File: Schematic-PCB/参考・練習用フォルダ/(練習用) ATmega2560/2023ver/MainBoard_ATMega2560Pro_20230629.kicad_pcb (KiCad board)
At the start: 2 copper layers, 70 x 103 mm, 43 parts, among them J1 Conn_01x10_Pin, J2 Conn_01x08_Male, J3 Conn_01x04_Female, J4 Conn_01x08_Male, J5 Conn_01x02_Male, J6 Conn_01x20_Male, J7 Conn_01x26_Male, J8 Conn_01x03_Pin, SW1 SW_DPST_x2, SW2 SW_DPST_x2, SW3 SW_DPST_x2, SW4 SW_DPDT_x2, U1 ATMEGA2560_pro

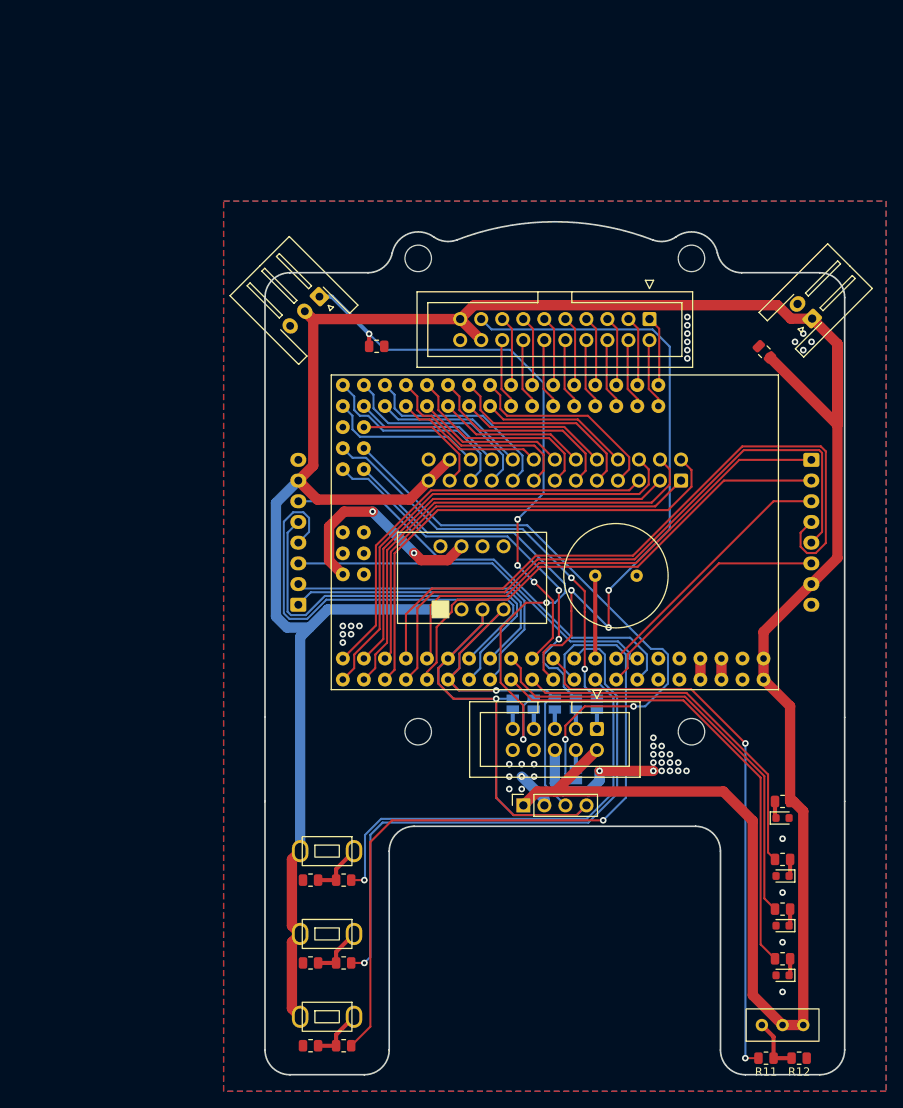
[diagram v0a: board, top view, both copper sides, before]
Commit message: update: いろいろなKiCadファイルを開いた
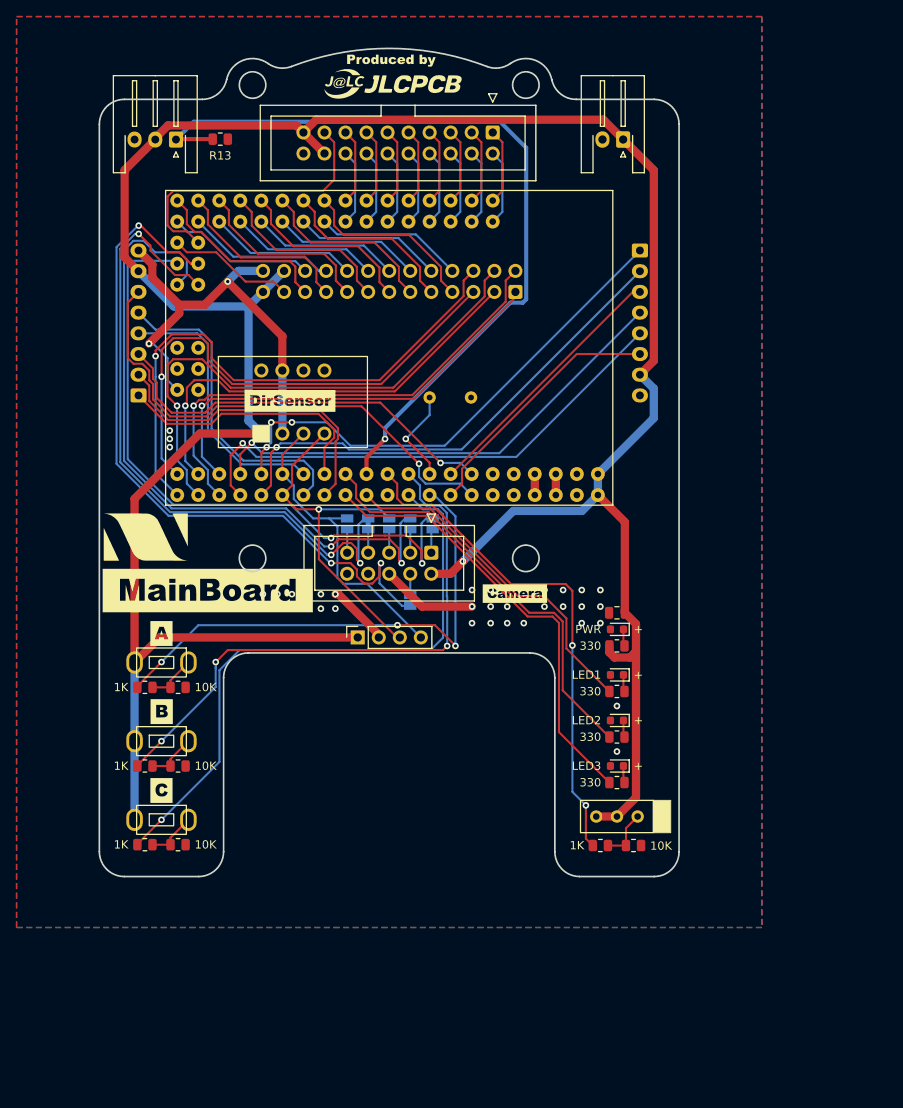
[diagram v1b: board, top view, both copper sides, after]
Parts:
- removed D1, D2, D3, D4: LED, LED_SMD:LED_0603_1608Metric
- removed REF** (x4): MountingHole_3.2mm_M3, MountingHole:MountingHole_3.2mm_M3
- added LED1: LED, LED_SMD:LED_0603_1608Metric, F.Cu at (112.5, 119.5)
- added LED2: LED, LED_SMD:LED_0603_1608Metric, F.Cu at (112.5, 125.0)
- added LED3: LED, LED_SMD:LED_0603_1608Metric, F.Cu at (112.5, 130.5)
- added PWR: LED, LED_SMD:LED_0603_1608Metric, F.Cu at (112.5, 114.0)
- BZ1: moved to B.Cu
- JP3: value Jumper_2_Open -> Jumper_2_Bridged; footprint Jumper:SolderJumper-2_P1.3mm_Open_Pad1.0x1.5mm -> Jumper:SolderJumper-2_P1.3mm_Bridged_Pad1.0x1.5mm
- moved C1 36.2 mm to (112.5, 112.0), turned to 180 degrees
- moved R9 34.1 mm to (55.5, 140.0), turned to 180 degrees
- moved R7 33.8 mm to (55.5, 130.5), turned to 180 degrees
- moved R5 33.4 mm to (55.5, 121.0), turned to 180 degrees
- moved J4 32.7 mm to (115.3, 68.2)
- moved R11 32.5 mm to (110.5, 140.1)
- moved R12 32.5 mm to (114.5, 140.1)
- moved SW4 32.2 mm to (112.5, 136.6), turned to 0 degrees
- moved J2 31.8 mm to (54.7, 85.8)
- moved J5 31.4 mm to (113.2, 54.9), turned to 180 degrees
- moved R13 31.3 mm to (64.6, 54.8)
- moved SW3 31.1 mm to (57.5, 137.0)
- moved SW2 30.7 mm to (57.5, 127.5)
- moved J7 30.3 mm to (100.2, 73.3)
- moved SW1 30.3 mm to (57.5, 118.0)
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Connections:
- U1 pad D11: Sig_NeoPixel -> unconnected-(U1-PadD11)
- U1 pad D48: unconnected-(U1-PadD48) -> Sig23_BALL-Kicker
- U1 pad D49: Sig23_BALL-Kicker -> Sig_NeoPixel
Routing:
- net VIN: track 376.9 -> 325.1 mm, vias 0 -> 1
- net SDA: track 88.2 -> 37.6 mm, vias 1 -> 0
- net Sig_NeoPixel: track 80.9 -> 35.2 mm, vias 3 -> 0
- net SCK: track 48.4 -> 84.4 mm
- net MISO: track 50.0 -> 77.9 mm
- net Sig_Kicker: track 70.3 -> 97.2 mm, vias 4 -> 1
- net GND: track 48.9 -> 74.2 mm, vias 46 -> 38
- net Sig_M4-1: track 83.1 -> 58.8 mm, vias 0 -> 1
- net Sig_M2-1: track 56.3 -> 33.1 mm
- net SS: track 60.9 -> 81.0 mm, vias 2 -> 3
- net Sig_M4-2: track 77.5 -> 62.2 mm, vias 0 -> 1
- net SCL: track 57.5 -> 43.3 mm
- net MOSI: track 72.5 -> 86.6 mm, vias 2 -> 3
- net Sig_BTN3: track 87.8 -> 73.8 mm
- net Sig_M2-2: track 52.1 -> 38.6 mm
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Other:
- board size 70 x 103 mm -> 70 x 100 mm
- board text added: "+"
- board text added: "10K"
- board text added: "1K"
- board text added: "330"
